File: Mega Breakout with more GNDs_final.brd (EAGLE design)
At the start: 101.6 x 61.9 mm, 13 parts

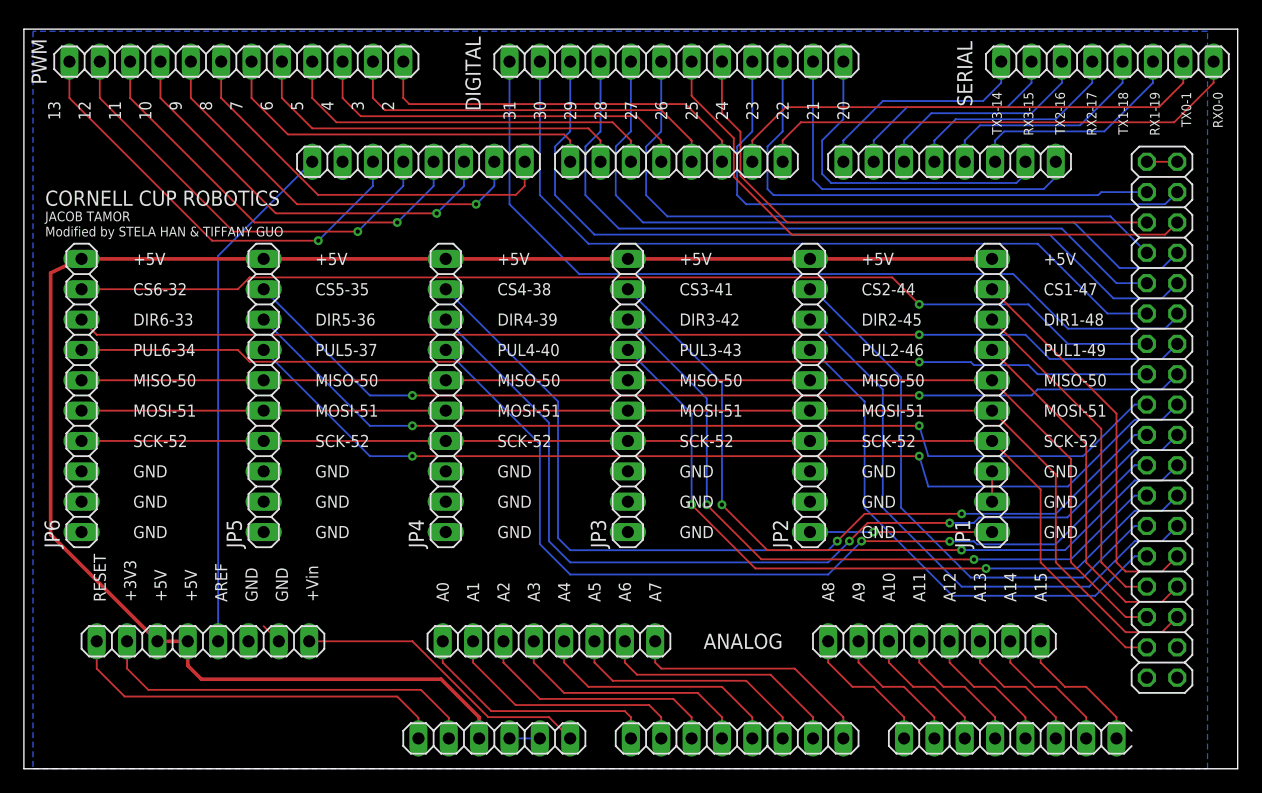
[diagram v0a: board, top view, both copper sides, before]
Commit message: final ver of modified PCB
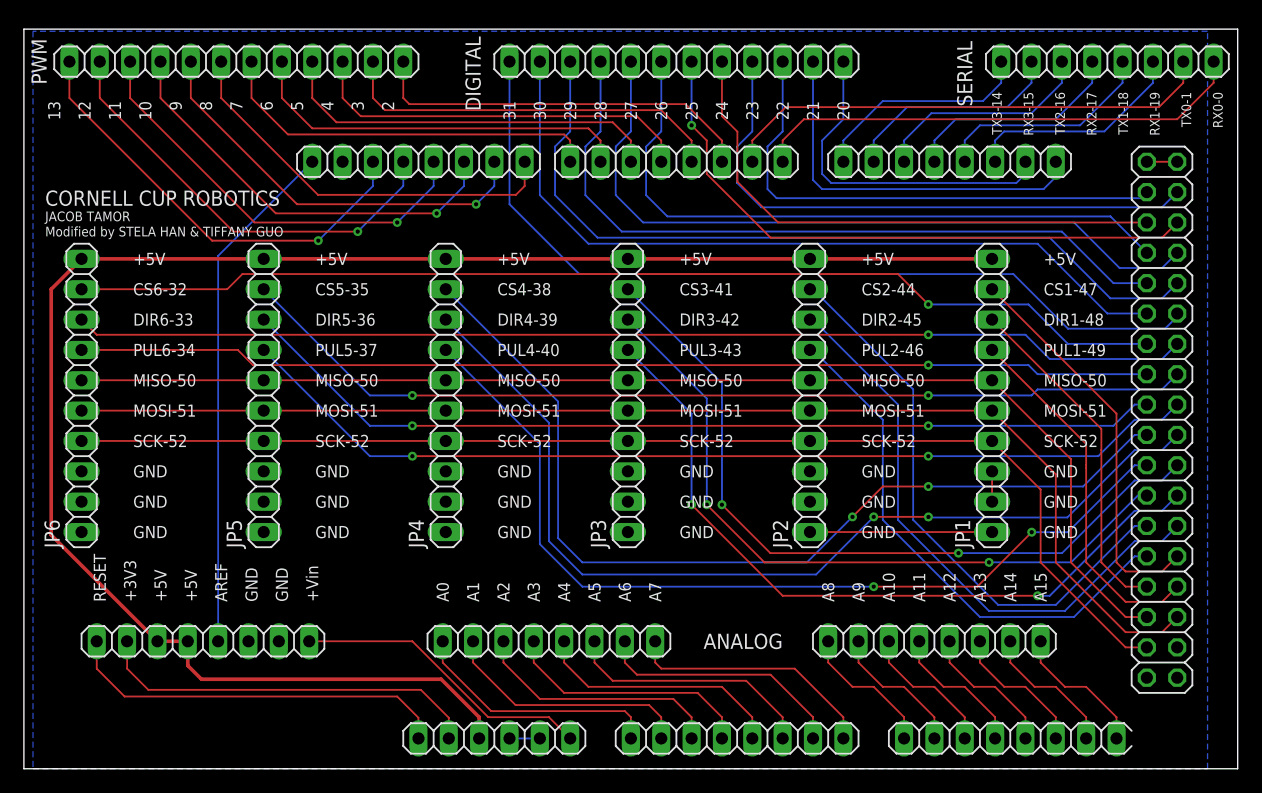
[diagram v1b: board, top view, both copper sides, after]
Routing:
- net PUL5-37: track 84.9 -> 81.9 mm
- net DIR5-36: track 81.3 -> 78.3 mm
- net CS2-44: track 46.4 -> 48.3 mm
- net PUL3-43: track 60.5 -> 62.4 mm
- net GND: track 22.1 -> 20.3 mm, vias 1 -> 0
- net DIR2-45: track 47.9 -> 49.4 mm
- net 25: track 50.6 -> 52.0 mm, vias 0 -> 1
- net +5V: track 146.8 -> 145.5 mm
- net PUL2-46: track 43.3 -> 44.5 mm
- net DIR4-39: track 79.9 -> 80.7 mm
- net CS4-38: track 78.4 -> 79.3 mm
- net PUL4-40: track 75.4 -> 76.0 mm
